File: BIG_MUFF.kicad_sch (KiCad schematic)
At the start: 58 parts, among them J1 9V DC, J2 IN, J3 OUT, J4 PINHD_1x3_Female, J5 PINHD_1x3_Male, Q1 BC547, Q2 BC547, Q3 BC547, Q4 BC547, SW6 SW_3PDT_Footswitch

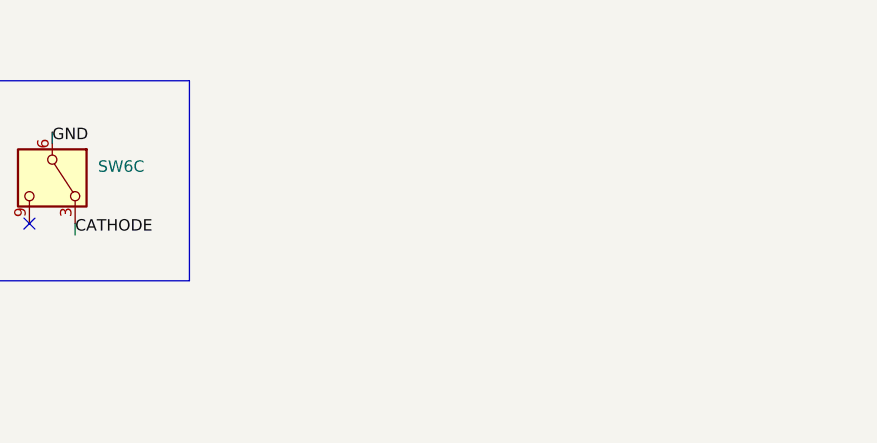
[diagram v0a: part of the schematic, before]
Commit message: DRM fix
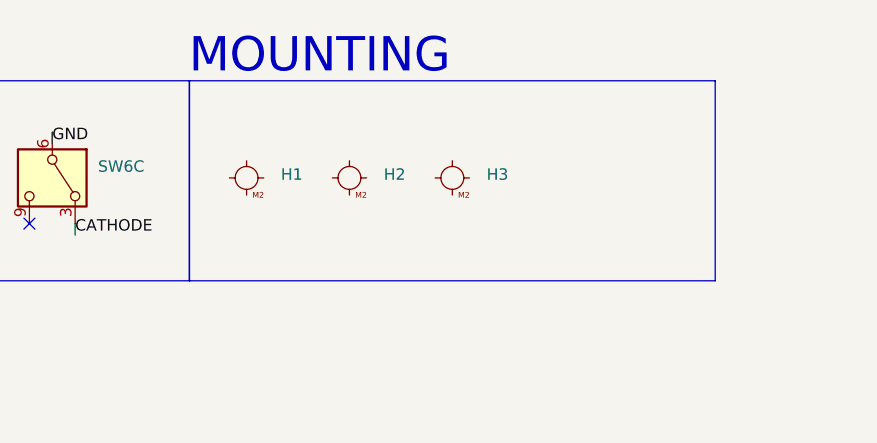
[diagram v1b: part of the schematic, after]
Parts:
- added H1, H2, H3: ~, PCM_fab:MountingHole_M2, symbol PCM_fab:MountingHole_M2
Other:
- note added: "MOUNTING"
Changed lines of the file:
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@@
 		)
 	)
+	(rectangle
+		(start 243.84 43.815)
+		(end 302.26 66.04)
+		(stroke
+			(width 0)
+			(type default)
+		)
+		(fill
+			(type none)
+		)
+	)
 	(text "Recovery Amp"
 		(exclude_from_sim no)
@@
 		)
 	)
+	(text "MOUNTING"
+		(exclude_from_sim no)
+		(at 258.318 41.148 0)
+		(effects
+			(font
+				(size 3.81 3.81)
+			)
+		)
+	)
 	(text "STAGE 2\n"
 		(exclude_from_sim no)
@@
 	)
 	(symbol
+		(lib_id "PCM_fab:MountingHole_M2")
+		(at 261.62 54.61 0)
+		(unit 1)
+		(exclude_from_sim no)
+		(in_bom yes)
+		(on_board yes)
+		(dnp no)
+		(fields_autoplaced yes)
+		(property "Reference" "H2"
+			(at 265.43 54.2303 0)
+			(effects
+				(font
+					(size 1.27 1.27)
+				)
+				(justify left)
+			)
+		)
+		(property "Value" "~"
+			(at 265.43 56.1354 0)
+			(effects
+				(font
+					(size 1.27 1.27)
+				)
+				(justify left)
+			)
+		)
+		(property "Footprint" "PCM_fab:MountingHole_M2"
+			(at 261.62 54.61 0)
+			(effects
+				(font
+					(size 1.27 1.27)
+				)
+				(hide yes)
+			)
+		)
+		(property "Datasheet" ""
+			(at 261.62 54.61 0)
+			(effects
+				(font
+					(size 1.27 1.27)
+				)
+				(hide yes)
+			)
+		)
+		(property "Description" ""
+			(at 261.62 54.61 0)
+			(effects
+				(font
+					(size 1.27 1.27)
+				)
+				(hide yes)
+			)
+		)
+		(instances
+			(project "BIG_MUFF"
+				(path "/00000000-0000-0000-0000-000000000001"
+					(reference "H2")
+					(unit 1)
+				)
+			)
+		)
+	)
+	(symbol
 		(lib_id "Transistor_BJT:BC547")
 		(at 68.58 144.78 90)
@@
 	)
 	(symbol
+		(lib_id "PCM_fab:MountingHole_M2")
+		(at 250.19 54.61 0)
+		(unit 1)
+		(exclude_from_sim no)
+		(in_bom yes)
+		(on_board yes)
+		(dnp no)
+		(fields_autoplaced yes)
+		(property "Reference" "H1"
+			(at 254 54.2303 0)
+			(effects
+				(font
+					(size 1.27 1.27)
+				)
+				(justify left)
+			)
+		)
+		(property "Value" "~"
+			(at 254 56.1354 0)
+			(effects
+				(font
+					(size 1.27 1.27)
+				)
+				(justify left)
+			)
+		)
+		(property "Footprint" "PCM_fab:MountingHole_M2"
+			(at 250.19 54.61 0)
+			(effects
+				(font
+					(size 1.27 1.27)
+				)
+				(hide yes)
+			)
+		)
+		(property "Datasheet" ""
+			(at 250.19 54.61 0)
+			(effects
+				(font
+					(size 1.27 1.27)
+				)
+				(hide yes)
+			)
+		)
+		(property "Description" ""
+			(at 250.19 54.61 0)
+			(effects
+				(font
+					(size 1.27 1.27)
+				)
+				(hide yes)
+			)
+		)
+		(instances
+			(project ""
+				(path "/00000000-0000-0000-0000-000000000001"
+					(reference "H1")
+					(unit 1)
+				)
+			)
+		)
+	)
+	(symbol
 		(lib_id "Device:D")
 		(at 115.57 137.16 0)
@@
 					(unit 1)
 				)
+			)
+		)
+	)
+	(symbol
+		(lib_id "PCM_fab:MountingHole_M2")
+		(at 273.05 54.61 0)
+		(unit 1)
+		(exclude_from_sim no)
+		(in_bom yes)
+		(on_board yes)
+		(dnp no)
+		(fields_autoplaced yes)
+		(property "Reference" "H3"
+			(at 276.86 54.2303 0)
+			(effects
+				(font
+					(size 1.27 1.27)
+				)
+				(justify left)
+			)
+		)
+		(property "Value" "~"
+			(at 276.86 56.1354 0)
+			(effects
+				(font
+					(size 1.27 1.27)
+				)
+				(justify left)
+			)
+		)
+		(property "Footprint" "PCM_fab:MountingHole_M2"
+			(at 273.05 54.61 0)
+			(effects
+				(font
+					(size 1.27 1.27)
+				)
+				(hide yes)
+			)
+		)
+		(property "Datasheet" ""
+			(at 273.05 54.61 0)
+			(effects
+				(font
+					(size 1.27 1.27)
+				)
+				(hide yes)
+			)
+		)
+		(property "Description" ""
+			(at 273.05 54.61 0)
+			(effects
+				(font
+					(size 1.27 1.27)
+				)
+				(hide yes)
+			)
+		)
+		(instances
+			(project "BIG_MUFF"
+				(path "/00000000-0000-0000-0000-000000000001"
+					(reference "H3")
+					(unit 1)
+				)
